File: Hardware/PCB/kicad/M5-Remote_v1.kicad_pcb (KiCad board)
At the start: 2 copper layers, 108.5 x 73.1 mm, 35 parts, among them M5-CORE2 M5Bus Header, SW1 PEL12T4225SS1024, SW2 PEL12T4225SS1024, SW3 PEL12T4225SS1024, SW4 PEL12T4225SS1024, U1 PCA9685PW, U2 MCP23017_SS, U3 CHERRY-MX-LED

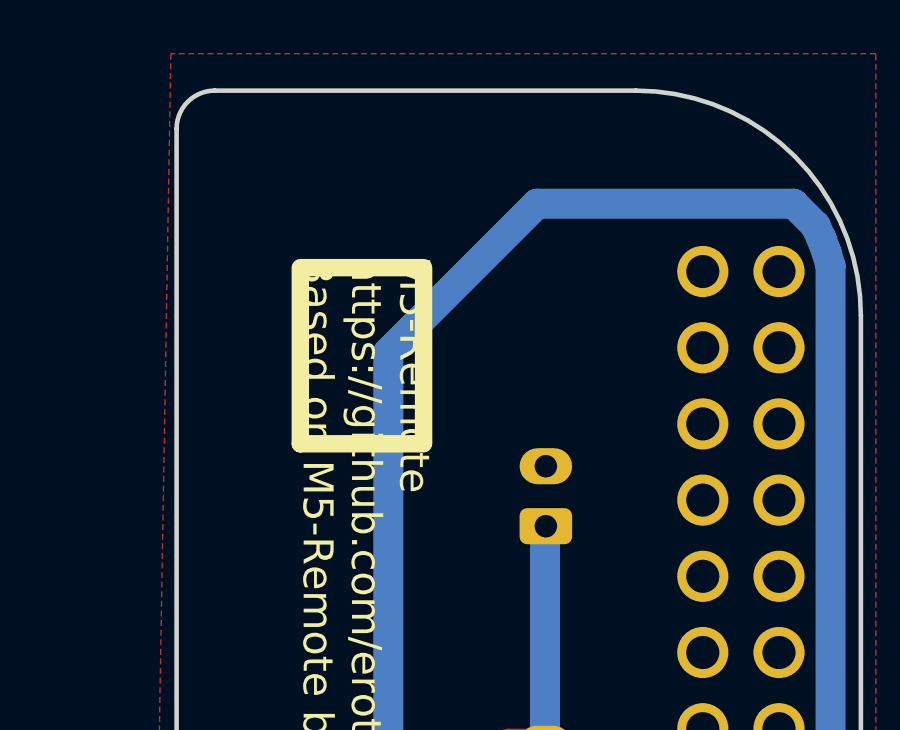
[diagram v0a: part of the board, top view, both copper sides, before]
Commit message: Tiny fix
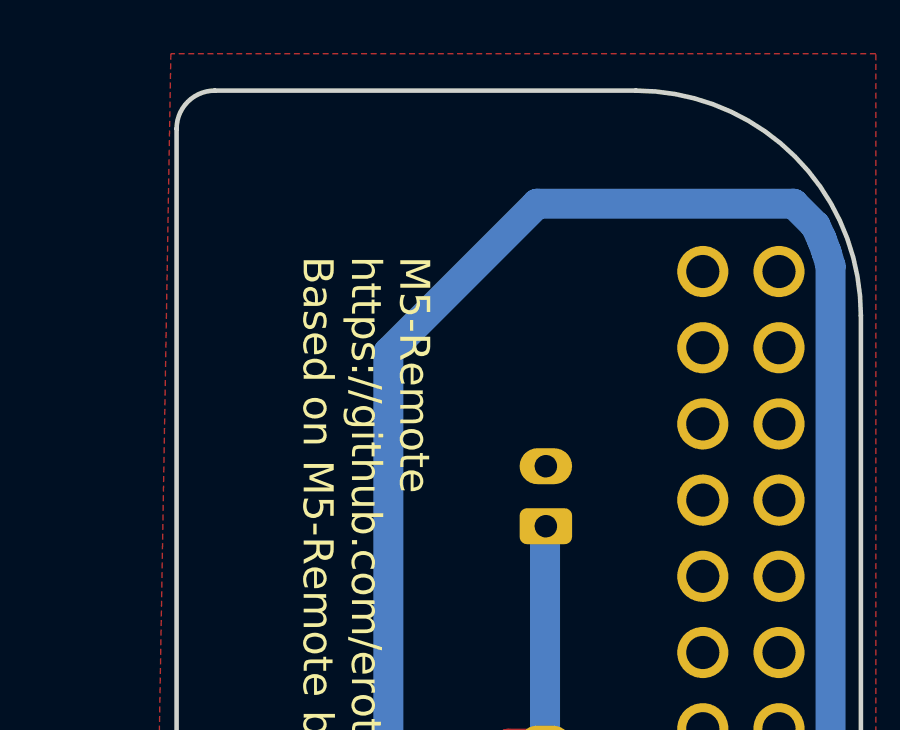
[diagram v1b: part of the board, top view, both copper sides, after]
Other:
- board text removed: ""
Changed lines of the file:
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@@
-		)
-	)
-	(gr_text ""
-		(at 151.933831 74.786 0)
-		(layer "F.SilkS")
-		(effects
-			(font
-				(size 5.870956 5.870956)
-				(thickness 0.580644)
-			)
-			(justify left)
 		)
 	)
